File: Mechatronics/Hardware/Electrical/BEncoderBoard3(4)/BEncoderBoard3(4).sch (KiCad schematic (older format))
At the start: 4 parts, among them J1 Conn_01x06_Male, U9 LSM6DSRX

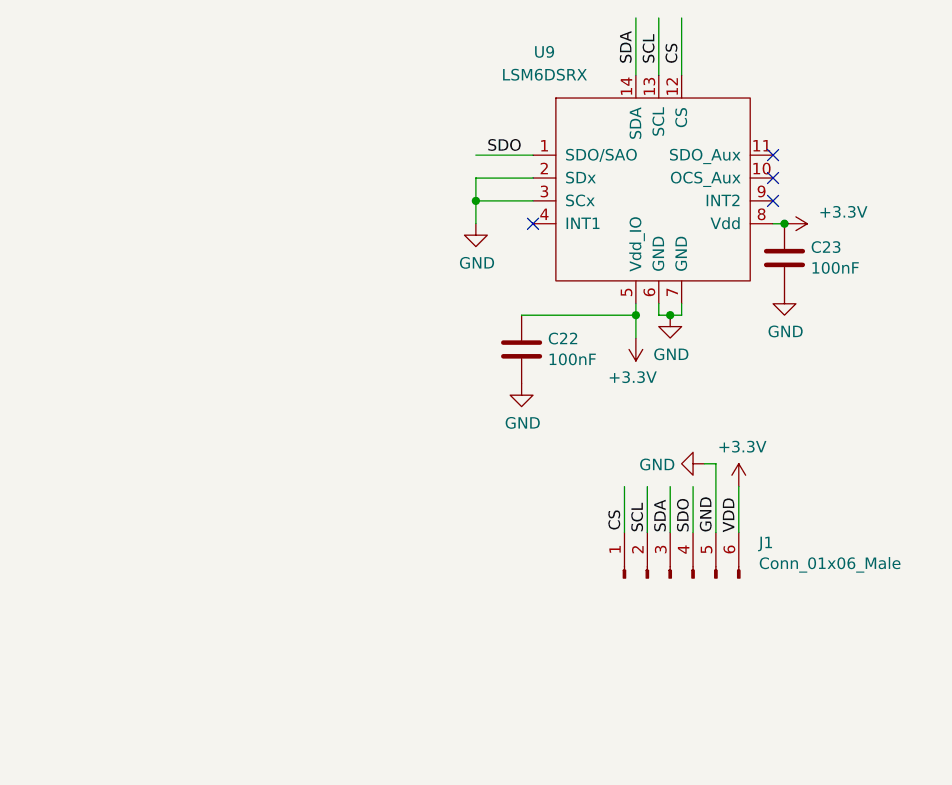
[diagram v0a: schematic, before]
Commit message: PCB changes
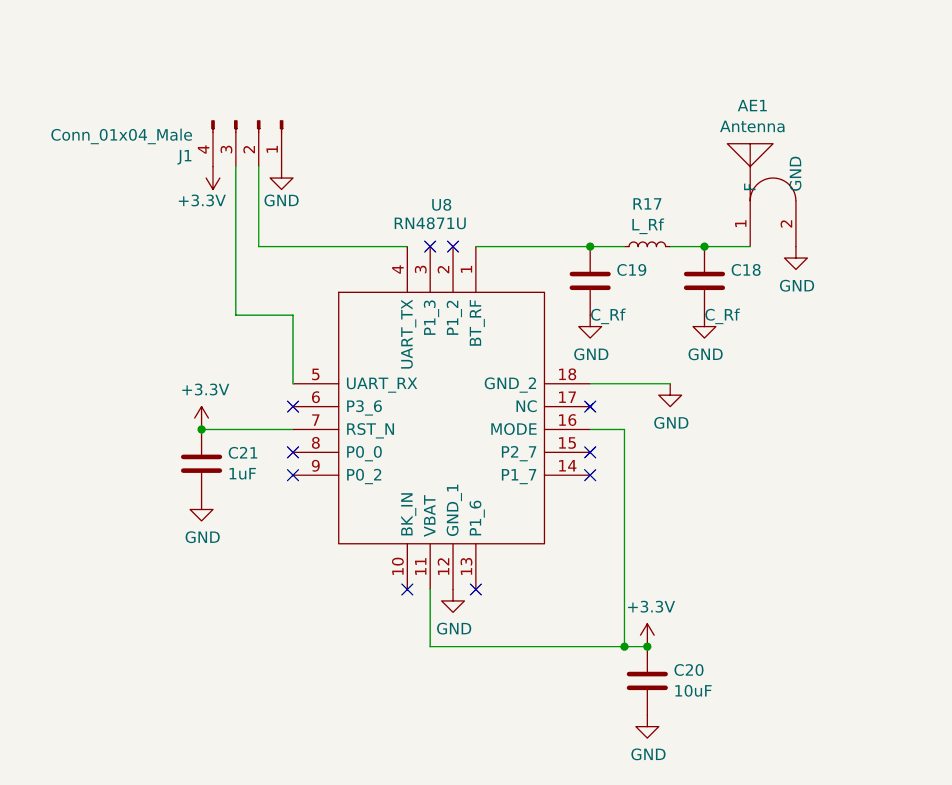
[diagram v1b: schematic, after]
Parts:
- removed C22, C23: 100nF, Encoder:C_0603_1608Metric_Pad1.05x0.95mm_HandSolder, symbol Device:C
- removed J1: Conn_01x06_Male, Encoder:SolderWirePad_1x06_SMD_5x10mm, symbol Connector:Conn_01x06_Male
- removed U9: LSM6DSRX, Encoder:LSM6DSRX, symbol Encoder:LSM6DSRX
- added AE1: Antenna, Encoder:Antenna, symbol Encoder:Antenna
- added C18, C19: C_Rf, Encoder:C_0402_1005Metric, symbol Device:C
- added C20: 10uF, Encoder:C_0603_1608Metric_Pad1.05x0.95mm_HandSolder, symbol Device:C
- added C21: 1uF, Encoder:C_0603_1608Metric_Pad1.05x0.95mm_HandSolder, symbol Device:C
- added J1: Conn_01x04_Male, Encoder:SolderWirePad_1x04_SMD_5x10mm_copy, symbol Connector:Conn_01x04_Male
- added R17: L_Rf, Encoder:L_0402_1005Metric, symbol Device:L_Small
- added U8: RN4871U, Encoder:RN4871U, symbol Encoder:RN4871U
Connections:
- net labels removed: CS, SCL, SDA, SDO, VDD
- wire segments 23 -> 16
- no-connect marks 4 -> 10
